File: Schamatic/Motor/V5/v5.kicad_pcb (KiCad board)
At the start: 2 copper layers, 47 parts, among them J1 SWD, J10 GND, J11 V, J12 U, J13 W, J2 SPI, J3 RS485, J4 RS485, J5 CAP+, J6 12, J7 12, J8 CAP-, J9 GND, Q1 PSMN3R3-40YS, Q2 PSMN3R3-40YS, Q3 PSMN3R3-40YS, Q4 PSMN3R3-40YS, Q5 PSMN3R3-40YS, Q6 PSMN3R3-40YS, SW1 SWiTCH, SW2 SWiTCH, U1 STSPIN32F0, U2 LTC2876, Y1 8Mhz

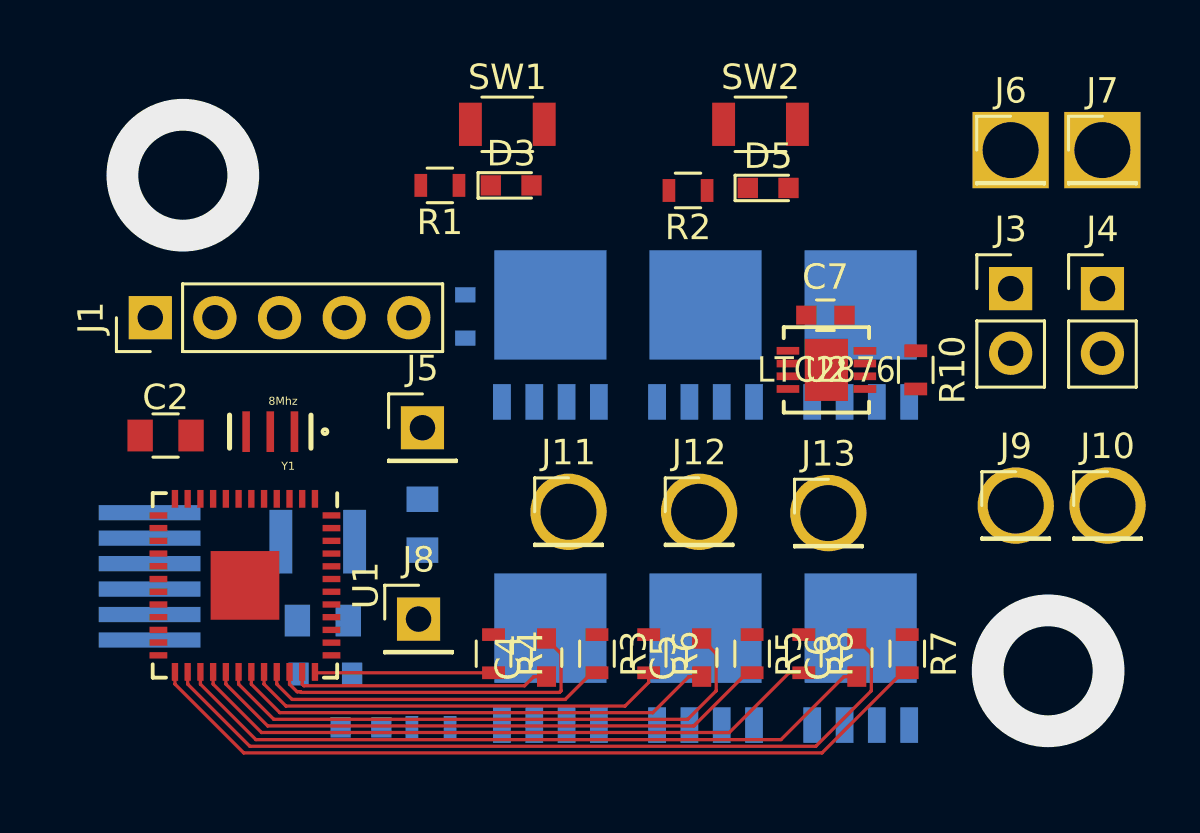
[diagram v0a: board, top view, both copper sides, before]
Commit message: trace done
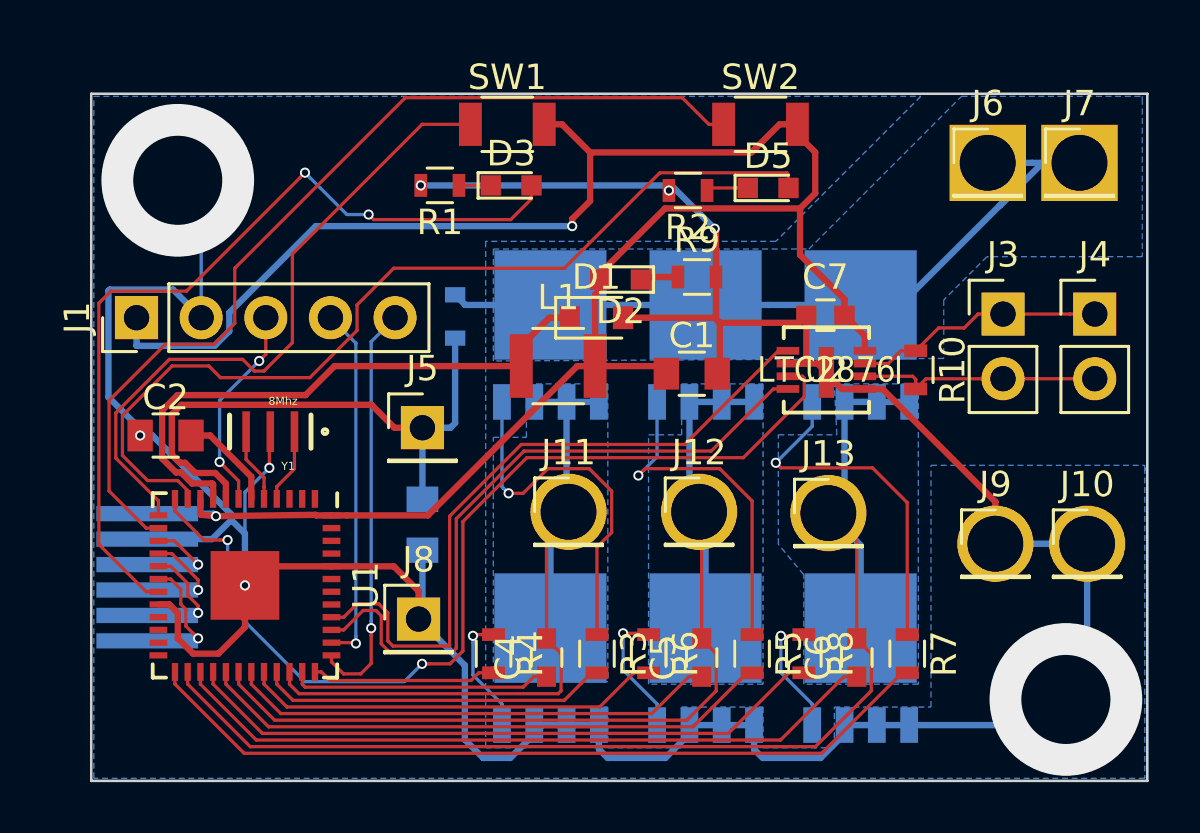
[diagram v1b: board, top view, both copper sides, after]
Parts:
- C1, D1, D2, L1, R9: moved to F.Cu
- moved R9 20.6 mm to (167.3, 97.2)
- moved D2 20.3 mm to (164.3, 97.3)
- moved D1 17.6 mm to (163.3, 98.8)
- moved C1 17.4 mm to (167.1, 101.0)
- moved L1 11.7 mm to (161.8, 100.7)
- moved J9 1.70 mm to (179.0, 107.7)
- moved J10 1.70 mm to (182.6, 107.7)
- moved J3 1.04 mm to (179.3, 98.7)
- moved J4 1.04 mm to (182.9, 98.7)
- moved J7 1.03 mm to (182.3, 92.7)
- moved J6 1.03 mm to (178.7, 92.7)
- moved J1 0.54 mm to (145.3, 98.8)
- moved D4 0.40 mm to (157.8, 98.8)
- moved J2 0.10 mm to (148.7, 108.8)
- turned C3 to 270 degrees
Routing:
- net Earth: track 0.00 -> 134.8 mm, vias 1 -> 8
- net +3V3: track 0.00 -> 81.7 mm, vias 0 -> 2
- net DE: track 0.00 -> 38.5 mm, vias 0 -> 2
- net Net-(SW2-Pad1): track 0.00 -> 36.9 mm
- net Net-(D5-Pad2): track 0.00 -> 36.7 mm
- net Net-(D3-Pad2): track 0.00 -> 33.3 mm, vias 0 -> 2
- net +12V: track 0.00 -> 31.2 mm
- net RX: track 0.00 -> 27.3 mm
- net TX: track 0.00 -> 26.9 mm
- net Net-(SW1-Pad1): track 0.00 -> 25.8 mm
- net Net-(D1-Pad1): track 0.00 -> 22.9 mm, vias 1 -> 0
- net VM: track 0.00 -> 22.7 mm
- net O3: track 31.5 -> 49.2 mm
- net O1: track 13.6 -> 30.7 mm
- net O2: track 22.6 -> 39.3 mm
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- added copper zone on B.Cu, net +12V
- added copper zone on B.Cu, net Earth
- added copper zone on B.Cu, net O1
- added copper zone on B.Cu, net O2
- added copper zone on B.Cu, net O3
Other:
- board outline added: 41.5 x 27 mm

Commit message: new board version ready to order
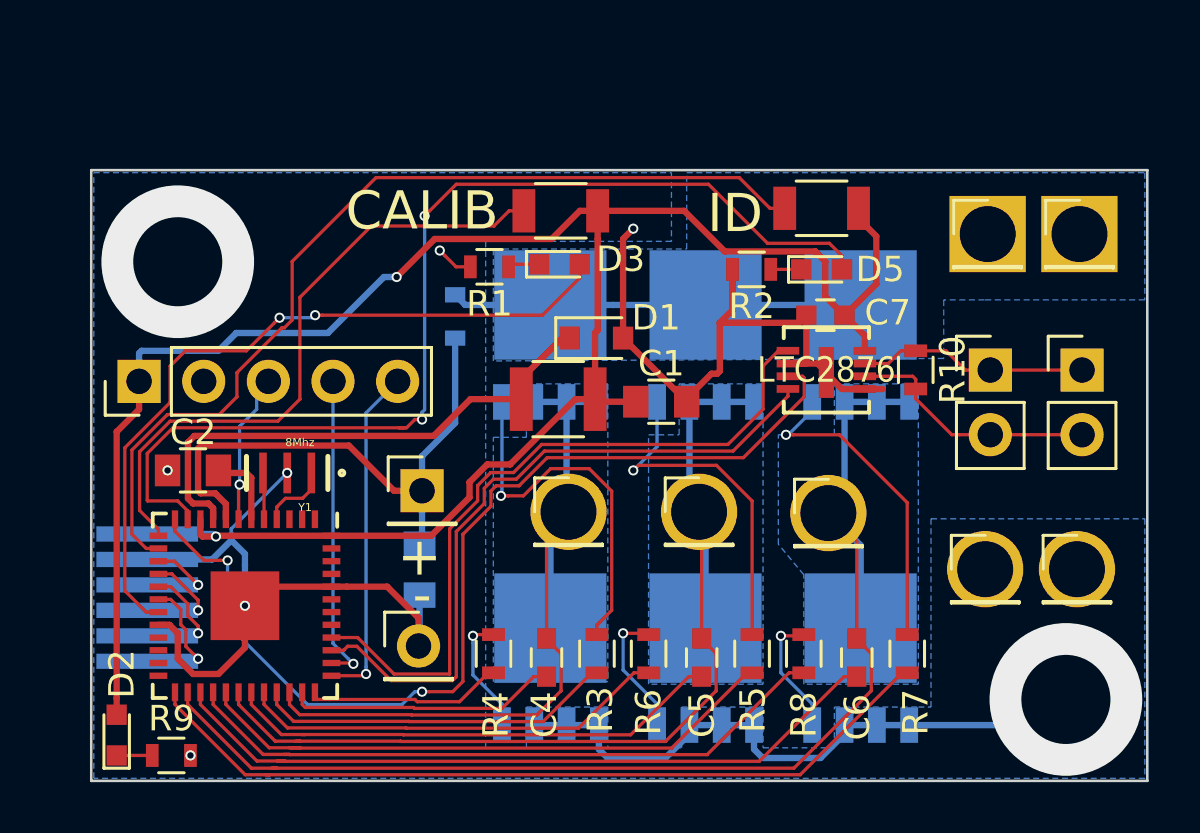
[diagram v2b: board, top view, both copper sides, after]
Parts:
- moved R9 27.9 mm to (146.7, 116.0)
- moved D2 26.7 mm to (144.5, 115.2), turned to 90 degrees
- moved ID 4.08 mm to (172.2, 94.5)
- moved CALIB 4.00 mm to (161.9, 94.6)
- moved R2 3.98 mm to (169.4, 96.9)
- moved D5 3.83 mm to (172.2, 96.9)
- moved R1 3.75 mm to (159.2, 96.8)
- moved D3 3.64 mm to (161.9, 96.7)
- moved J6 2.80 mm to (178.7, 95.5)
- moved J7 2.80 mm to (182.3, 95.5)
- moved J1 2.50 mm to (145.4, 101.3)
- moved + 2.48 mm to (156.5, 105.6)
- moved B 2.26 mm to (182.4, 100.9)
- moved J3 2.26 mm to (178.8, 100.9)
- moved C3 1.77 mm to (156.4, 108.7)
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- renumbered J5 to +, J8 to -, J4 to B, SW1 to CALIB, SW2 to ID
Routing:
- net Earth: track 134.8 -> 79.6 mm
- net +12V: track 31.2 -> 17.7 mm
- net Net-(D5-Pad2): track 36.7 -> 42.2 mm, vias 0 -> 2
- net Net-(D3-Pad2): track 33.3 -> 29.3 mm
- net SWDIO: track 16.2 -> 13.4 mm
- net +3V3: track 81.7 -> 84.1 mm
- net NRST: track 8.18 -> 5.90 mm, vias 2 -> 1
- net Net-(D1-Pad1): track 22.9 -> 21.0 mm
- net SWDCLK: track 14.2 -> 12.3 mm
- net RX: track 27.3 -> 28.5 mm
- net DE: track 38.5 -> 39.7 mm
- net Net-(Q5-Pad4): track 14.0 -> 12.8 mm
- net Net-(U1-Pad5): track 2.93 -> 1.83 mm
- net Net-(C2-Pad2): track 3.91 -> 3.00 mm
- net VM: track 22.7 -> 21.8 mm
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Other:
- board size 41.5 x 27 mm -> 41.5 x 24 mm
- board text added: "+"
- board text added: "-"
- board text added: "3v3"
- board text added: "CS"
- board text added: "GND"
- board text added: "IO"
- board text added: "MISO"
- board text added: "MOSI"
- board text added: "NRST"
- board text added: "SCK"
- board text added: "SWDCLK"
